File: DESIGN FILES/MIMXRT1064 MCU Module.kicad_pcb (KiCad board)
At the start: 2 copper layers, 22 x 62 mm, 67 parts, among them J601 TF-15x15, U401 MIMXRT1064CVL5B, U601 IS25WP064A-JBLE, U602 IS42S16160J-6BLI, U701 M.2-B-KEY, Y401 7V24000026, Y402 Q13FC1350000200

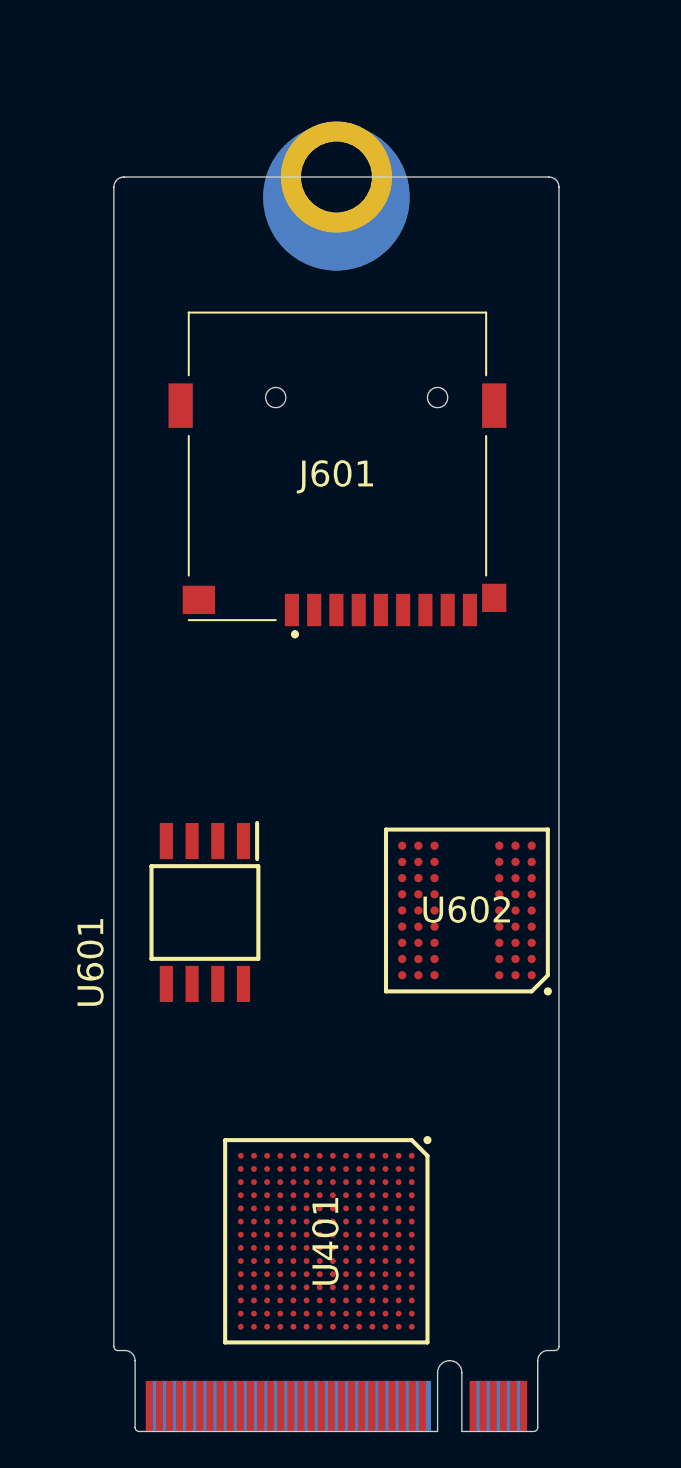
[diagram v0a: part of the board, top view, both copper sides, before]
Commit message: updates
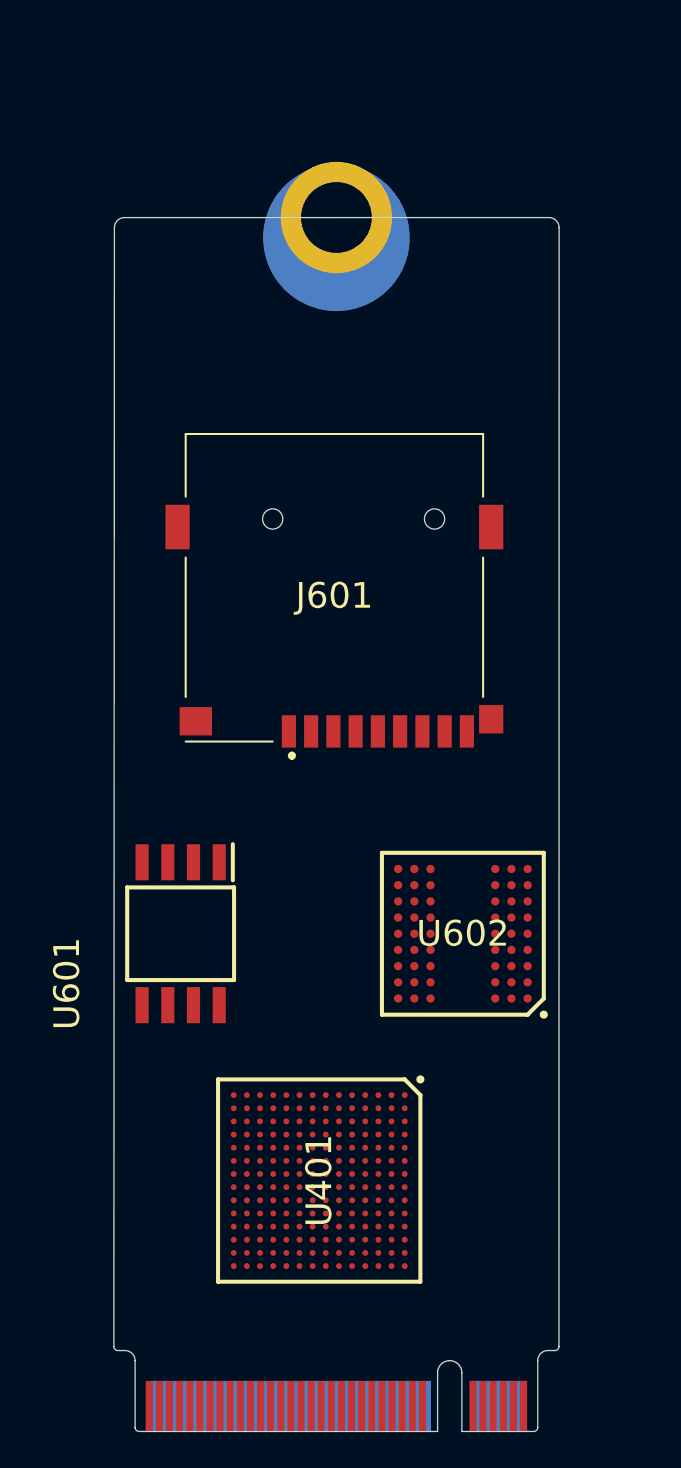
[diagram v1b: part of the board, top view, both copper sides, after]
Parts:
- moved J601 6.00 mm to (144.5, 90.7)
- moved U401 3.02 mm to (143.8, 120.0)
- moved U601 1.59 mm to (136.9, 107.8)
- moved U602 1.17 mm to (150.8, 107.8)
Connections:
- C510 pad 1: +5V -> VBUS
- U401 pad K14: MIDI_IN -> MIDI_OUT
- U401 pad L14: MIDI_OUT -> MIDI_IN
- U401 pad N6: +5V -> VBUS
- U701 pad MOUNTING-HOLE: unconnected-(U701-PadMOUNTING-HOLE) -> GND
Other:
- board size 22 x 62 mm -> 22 x 60 mm
- copper layers 2 -> 6
- board text removed: "1V8"
- board text removed: "RESET CIRCUIT"
